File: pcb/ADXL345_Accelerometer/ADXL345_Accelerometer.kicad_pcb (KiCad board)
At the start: 2 copper layers, 25.4 x 22.9 mm, 16 parts, among them J1 Conn_01x09, Q1 BSS138, Q2 BSS138, U1 ADXL345_Library, U2 AP2112K-3.3

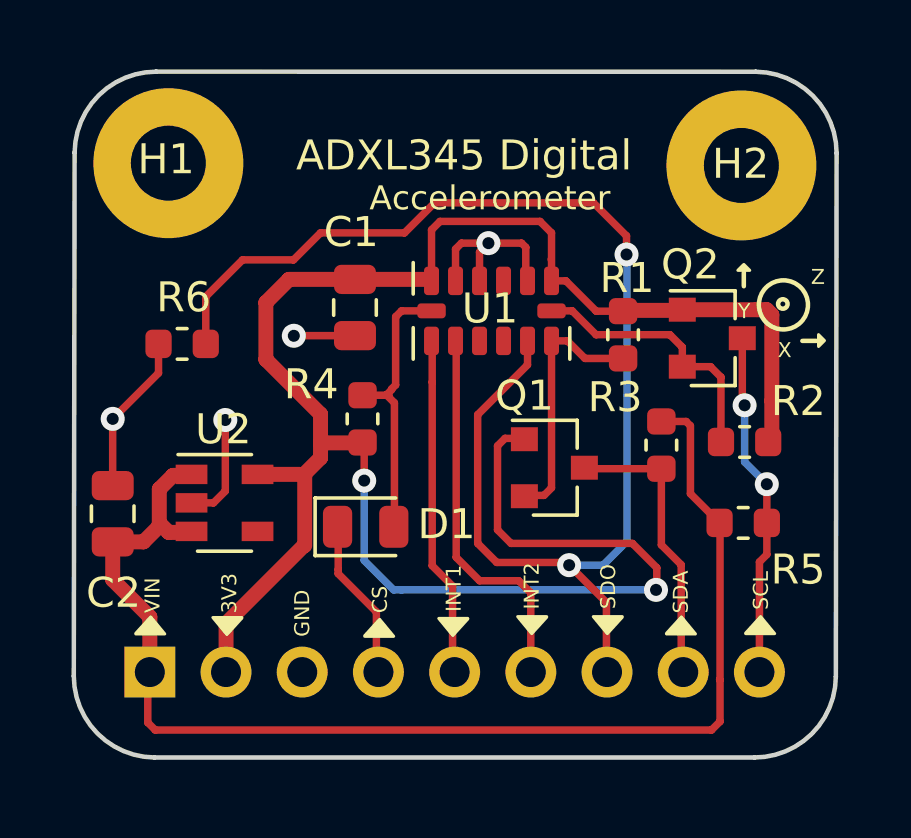
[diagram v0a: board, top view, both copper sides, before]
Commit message: Correcciones
Se corrigieron segun las recomendaciones realizadas por el docente.
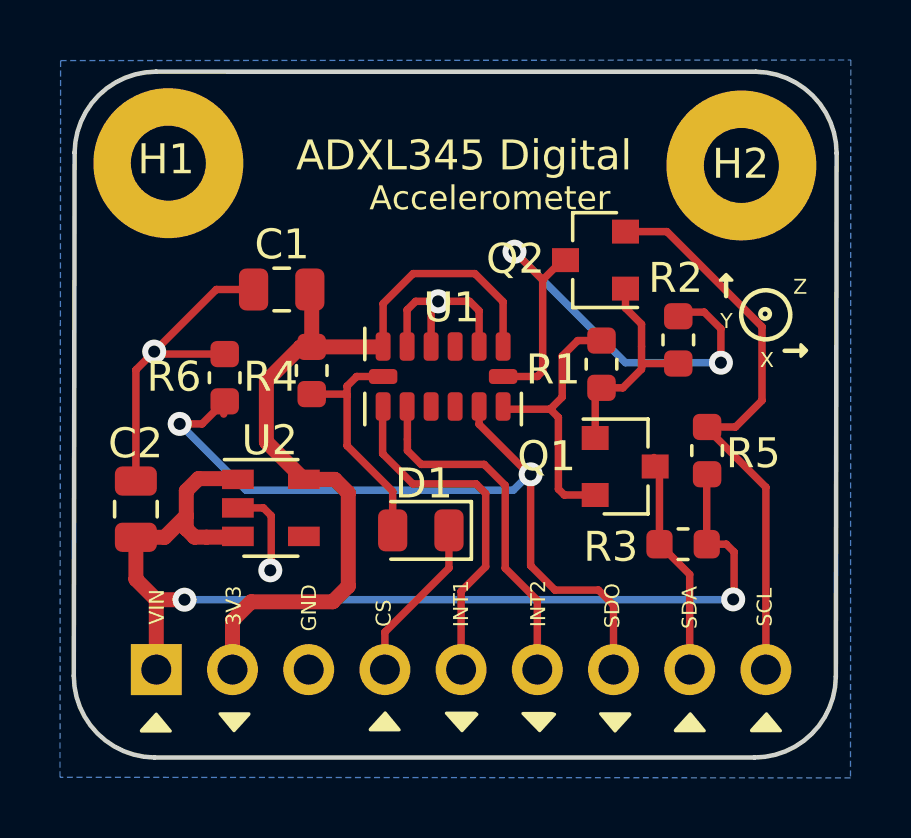
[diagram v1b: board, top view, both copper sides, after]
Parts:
- U1: value ADXL345_Library -> ADXL345
- moved Q2 4.68 mm to (148.6, 87.6), turned to 180 degrees
- moved R2 4.06 mm to (151.4, 90.3), turned to 270 degrees
- moved R3 3.38 mm to (151.6, 97.1), turned to 180 degrees
- moved U1 2.72 mm to (143.6, 91.5)
- moved R5 2.69 mm to (152.3, 94.0), turned to 270 degrees
- moved C1 2.52 mm to (138.2, 88.6), turned to 180 degrees
- moved Q1 2.36 mm to (149.6, 94.5)
- moved R4 2.34 mm to (139.2, 91.3), turned to 270 degrees
- moved D1 1.84 mm to (142.8, 96.6), turned to 180 degrees
- moved R6 1.81 mm to (136.3, 91.5), turned to 90 degrees
- moved U2 1.56 mm to (137.8, 95.9)
- moved R1 1.22 mm to (148.8, 91.1), turned to 90 degrees
- moved C2 0.79 mm to (133.3, 95.9)
- moved J1 0.23 mm to (134.0, 101.3)
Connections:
- net /SDA\SDIO_3V renamed Net-(Q1-Pad2)
- C1 pad 1: +3V3 -> Net-(C1-Pad1)
- J1 pad 2: +3V3 -> Net-(C1-Pad1)
- Q2 pad 2: /SCL_3V -> /SCL
- Q2 pad 3: /SCL -> /SCL_3V
- R2 pad 1: +3V3 -> /SCL_3V
- R2 pad 2: /SCL_3V -> +3V3
- R4 pad 1: +3V3 -> Net-(C1-Pad1)
- R5 pad 1: /VIN -> /SCL
- R5 pad 2: /SCL -> /VIN
- U1 pad 1: +3V3 -> Net-(C1-Pad1)
- U1 pad 6: +3V3 -> Net-(C1-Pad1)
- U2 pad 5: +3V3 -> Net-(C1-Pad1)
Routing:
- net +3V3: track 67.4 -> 7.55 mm, vias 2 -> 0
- net Net-(C1-Pad1): track 0.00 -> 28.5 mm
- net /SDO\ADDR: track 44.7 -> 26.7 mm
- net /SCL_3V: track 9.29 -> 18.1 mm, vias 0 -> 2
- net /SCL: track 11.6 -> 19.7 mm, vias 2 -> 0
- net /VIN: track 42.5 -> 35.7 mm, vias 0 -> 2
- net GND: track 17.3 -> 20.8 mm, vias 5 -> 3
- net /SDA\SDIO: track 10.2 -> 7.64 mm
- net /INT2: track 12.8 -> 11.3 mm
- net /CS: track 6.42 -> 5.52 mm
- net Net-(Q1-Pad2): track 8.53 -> 9.15 mm
- net /INT1: track 11.9 -> 11.3 mm
- added copper zone on B.Cu, net GND
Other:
- net class Alimentacion: clearance 0.2 -> 0.4
- net class Default: clearance 0.2 -> 0.4
- rule trace_clearance: 0.2 -> 0.4
